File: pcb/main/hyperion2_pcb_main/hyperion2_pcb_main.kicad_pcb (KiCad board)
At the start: 2 copper layers, 6 parts, among them J1 RJ45_LED_Shielded, T1 H1102NLT, U1 ESP32-S3-WROOM-1U-N16R8, U2 MAX3488ECSA_, U3 PCA9685PW_118, U4 W5500

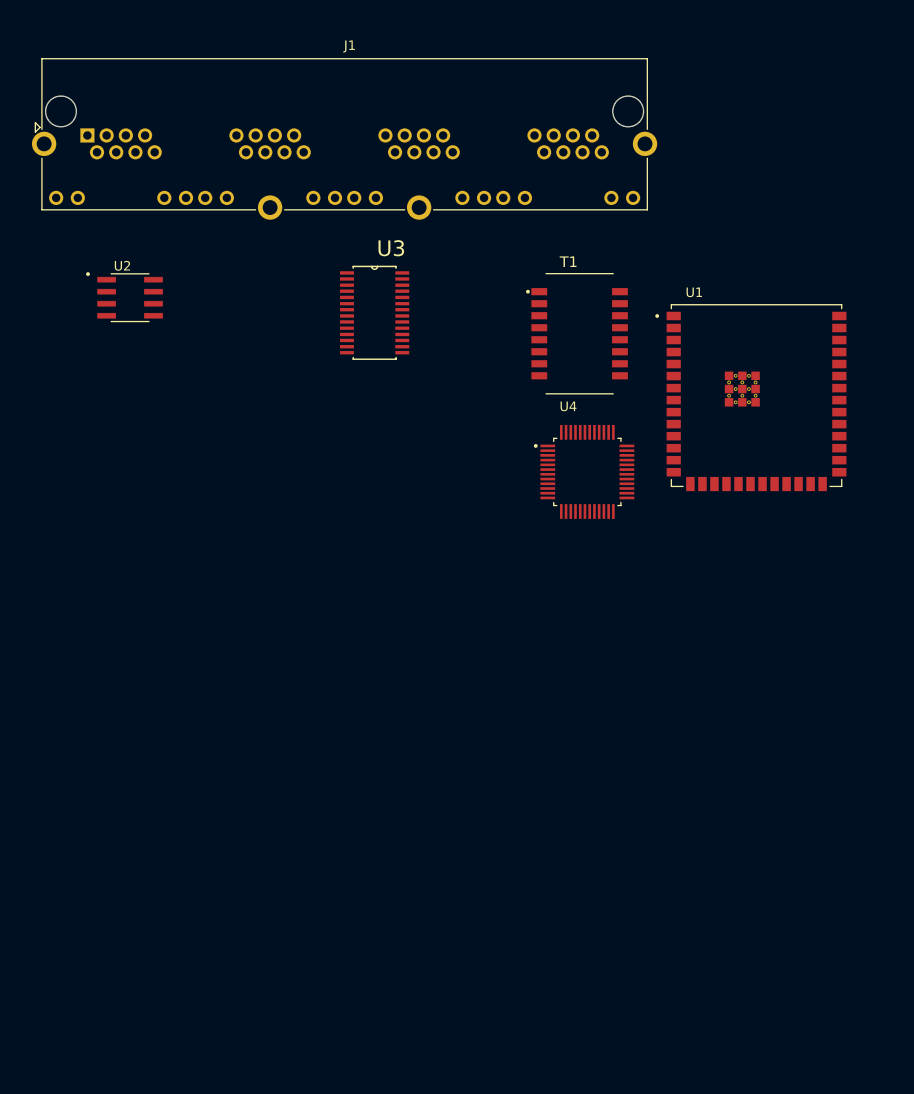
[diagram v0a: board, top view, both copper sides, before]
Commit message: placed more components
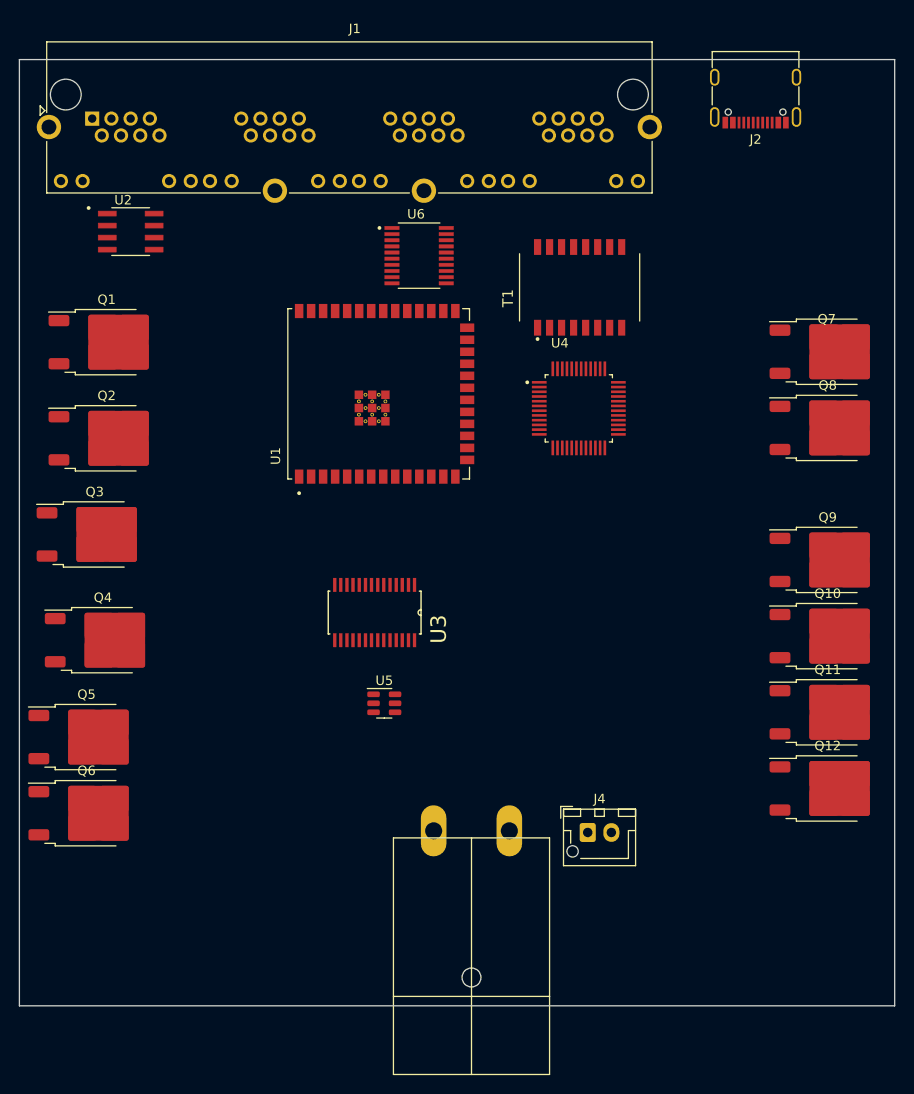
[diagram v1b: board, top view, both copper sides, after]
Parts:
- added J2: USB_C_Receptacle_USB2.0, Connector_USB:USB_C_Receptacle_G-Switch_GT-USB-7010ASV, F.Cu at (177.8, 27.9)
- added J3: Barrel_Jack, powerpole:POWERPOLEPCBMOUNT, F.Cu at (147.8, 124.0)
- added J4: Barrel_Jack, Connector_JST:JST_XH_B2B-XH-AM_1x02_P2.50mm_Vertical, F.Cu at (160.1, 106.7)
- added Q1: NCV8401, Package_TO_SOT_SMD:TO-252-2, F.Cu at (109.2, 54.9)
- added Q10: NCV8401, Package_TO_SOT_SMD:TO-252-2, F.Cu at (185.4, 85.9)
- added Q11: NCV8401, Package_TO_SOT_SMD:TO-252-2, F.Cu at (185.4, 94.0)
- added Q12: NCV8401, Package_TO_SOT_SMD:TO-252-2, F.Cu at (185.4, 102.0)
- added Q2: NCV8401, Package_TO_SOT_SMD:TO-252-2, F.Cu at (109.2, 65.0)
- added Q3: NCV8401, Package_TO_SOT_SMD:TO-252-2, F.Cu at (108.0, 75.2)
- added Q4: NCV8401, Package_TO_SOT_SMD:TO-252-2, F.Cu at (108.8, 86.4)
- added Q5: NCV8401, Package_TO_SOT_SMD:TO-252-2, F.Cu at (107.1, 96.6)
- added Q6: NCV8401, Package_TO_SOT_SMD:TO-252-2, F.Cu at (107.1, 104.7)
- added Q7: NCV8401, Package_TO_SOT_SMD:TO-252-2, F.Cu at (185.4, 55.9)
- added Q8: NCV8401, Package_TO_SOT_SMD:TO-252-2, F.Cu at (185.4, 63.9)
- added Q9: NCV8401, Package_TO_SOT_SMD:TO-252-2, F.Cu at (185.4, 77.9)
- added U5: LMR16006YQ5, Package_TO_SOT_SMD:SOT-23-6, F.Cu at (138.6, 93.0)
- added U6: SN74HCT245PWR, SN74HCT245PWR:SOP65P640X120-20N, F.Cu at (142.2, 45.7)
- moved U1 39.9 mm to (138.0, 60.3), turned to 90 degrees
- moved U3 31.7 mm to (137.5, 83.4), turned to -90 degrees
- moved U2 6.99 mm to (111.8, 43.2)
- moved U4 6.78 mm to (159.1, 61.9)
- moved T1 4.90 mm to (159.2, 49.1), turned to 90 degrees
- moved J1 1.85 mm to (107.7, 31.2)
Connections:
- J1 pad 37: unconnected-(J1D-1-Pad37) -> Net-(J1D-1)
- J1 pad 38: unconnected-(J1D-2-Pad38) -> Net-(J1D-2)
- J1 pad 39: unconnected-(J1D-3-Pad39) -> Net-(J1D-3)
- J1 pad 42: unconnected-(J1D-6-Pad42) -> Net-(J1D-6)
- T1 pad 1: unconnected-(T1-Pad1) -> Net-(U4-TXP)
- T1 pad 11: unconnected-(T1-Pad11) -> Net-(J1D-3)
- T1 pad 14: unconnected-(T1-Pad14) -> Net-(J1D-2)
- T1 pad 16: unconnected-(T1-Pad16) -> Net-(J1D-1)
- T1 pad 3: unconnected-(T1-Pad3) -> Net-(U4-TXN)
- T1 pad 6: unconnected-(T1-Pad6) -> Net-(U4-RXP)
- T1 pad 8: unconnected-(T1-Pad8) -> Net-(U4-RXN)
- T1 pad 9: unconnected-(T1-Pad9) -> Net-(J1D-6)
- U1 pad 13: unconnected-(U1-IO19-Pad13) -> Net-(U1-IO19)
- U1 pad 14: unconnected-(U1-IO20-Pad14) -> Net-(U1-IO20)
- U1 pad 17: unconnected-(U1-IO9-Pad17) -> Net-(U1-IO9)
- U1 pad 18: unconnected-(U1-IO10-Pad18) -> Net-(U1-IO10)
- U1 pad 19: unconnected-(U1-IO11-Pad19) -> Net-(U1-IO11)
- U1 pad 20: unconnected-(U1-IO12-Pad20) -> Net-(U1-IO12)
- U1 pad 21: unconnected-(U1-IO13-Pad21) -> Net-(U1-IO13)
- U1 pad 22: unconnected-(U1-IO14-Pad22) -> Net-(U1-IO14)
- U4 pad 1: unconnected-(U4-TXN-Pad1) -> Net-(U4-TXN)
- U4 pad 2: unconnected-(U4-TXP-Pad2) -> Net-(U4-TXP)
- U4 pad 32: unconnected-(U4-~{SCSN}-Pad32) -> Net-(U1-IO9)
- U4 pad 33: unconnected-(U4-SCLK-Pad33) -> Net-(U1-IO10)
- U4 pad 34: unconnected-(U4-MISO-Pad34) -> Net-(U1-IO11)
- U4 pad 35: unconnected-(U4-MOSI-Pad35) -> Net-(U1-IO12)
- U4 pad 36: unconnected-(U4-~{INTN}-Pad36) -> Net-(U1-IO13)
- U4 pad 37: unconnected-(U4-~{RSTN}-Pad37) -> Net-(U1-IO14)
- U4 pad 5: unconnected-(U4-RXN-Pad5) -> Net-(U4-RXN)
- U4 pad 6: unconnected-(U4-RXP-Pad6) -> Net-(U4-RXP)
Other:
- board outline added: 92.5 x 100 mm
- copper layers 2 -> 4
